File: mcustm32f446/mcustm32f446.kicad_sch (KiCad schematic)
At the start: 30 parts, among them J2 STM32WORLD_BASE, U1 AMS1117-3.3, U2 SRV05-4, U3 STM32F446RCTx, Y1 X_16MHZ

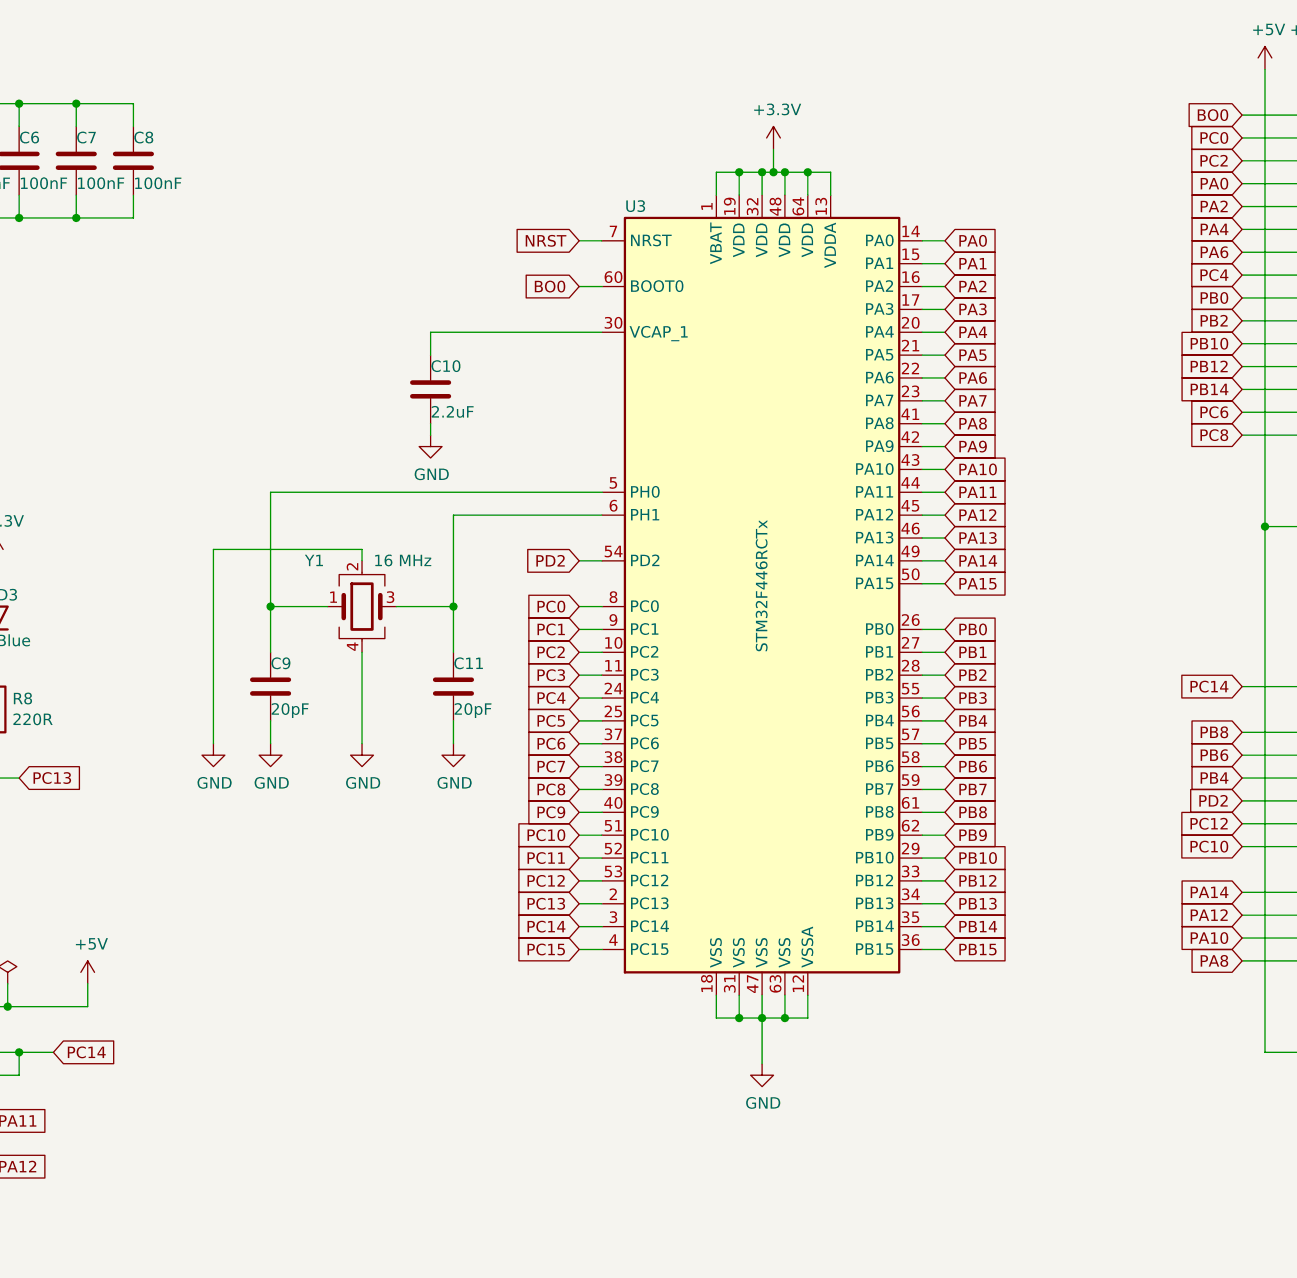
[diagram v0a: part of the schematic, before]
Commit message: Hmmmm
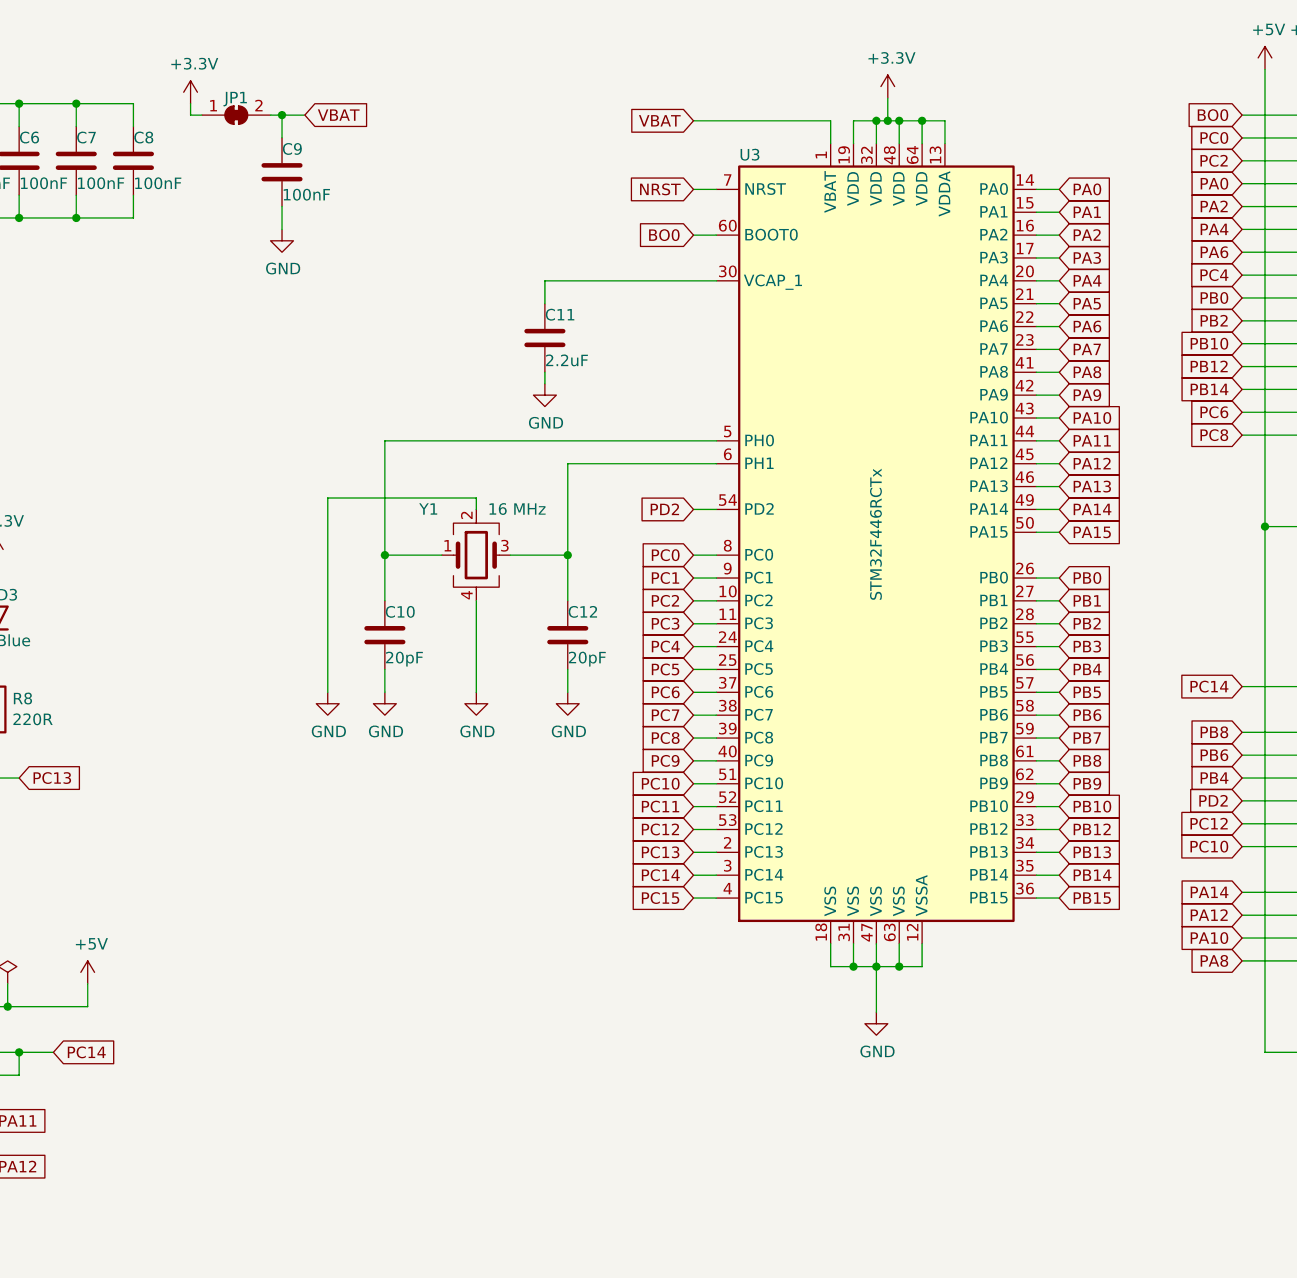
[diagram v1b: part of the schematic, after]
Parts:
- added C9: C_100NF_0603, Capacitor_SMD:C_0603_1608Metric, symbol stm32world:C_100NF_0603
- added JP1: ~, symbol Jumper:SolderJumper_2_Bridged
- renumbered C9 to C10, C10 to C11, C11 to C12
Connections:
- net +3V3: now also JP1.1 (A); no longer U3.1 (VBAT)
- net GND: now also C9.2
- new net VBAT: C9.1, JP1.2 (B), U3.1 (VBAT)
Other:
- moved on the sheet: C10, C11, C12, U3, Y1

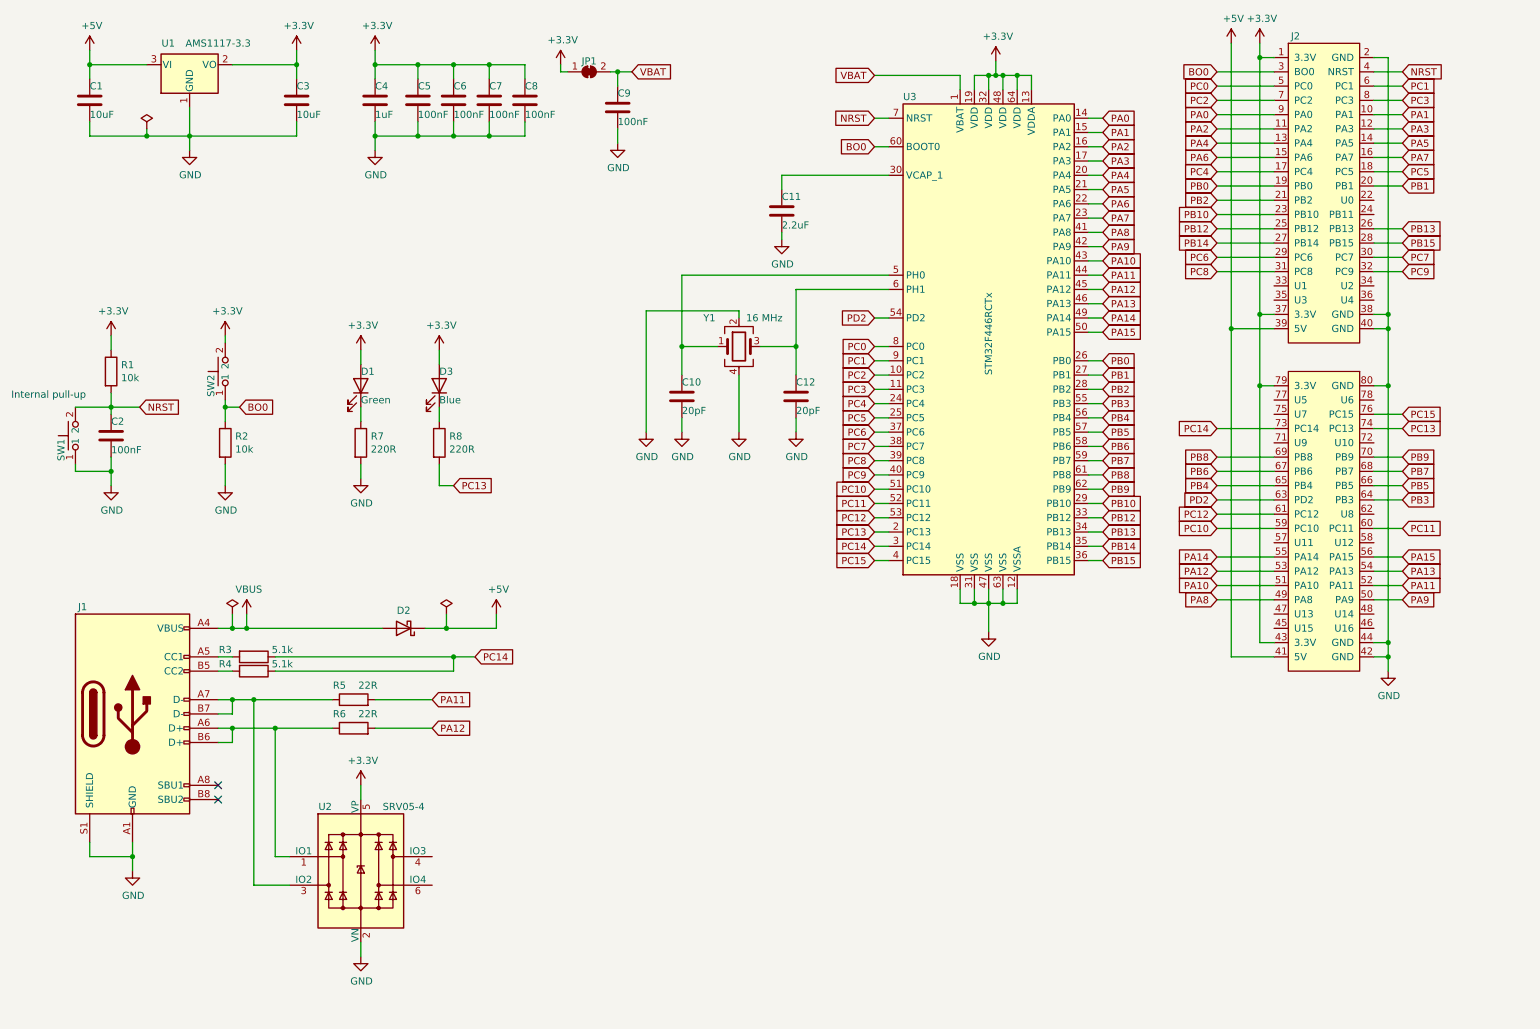
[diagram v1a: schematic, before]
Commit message: Hmmmm
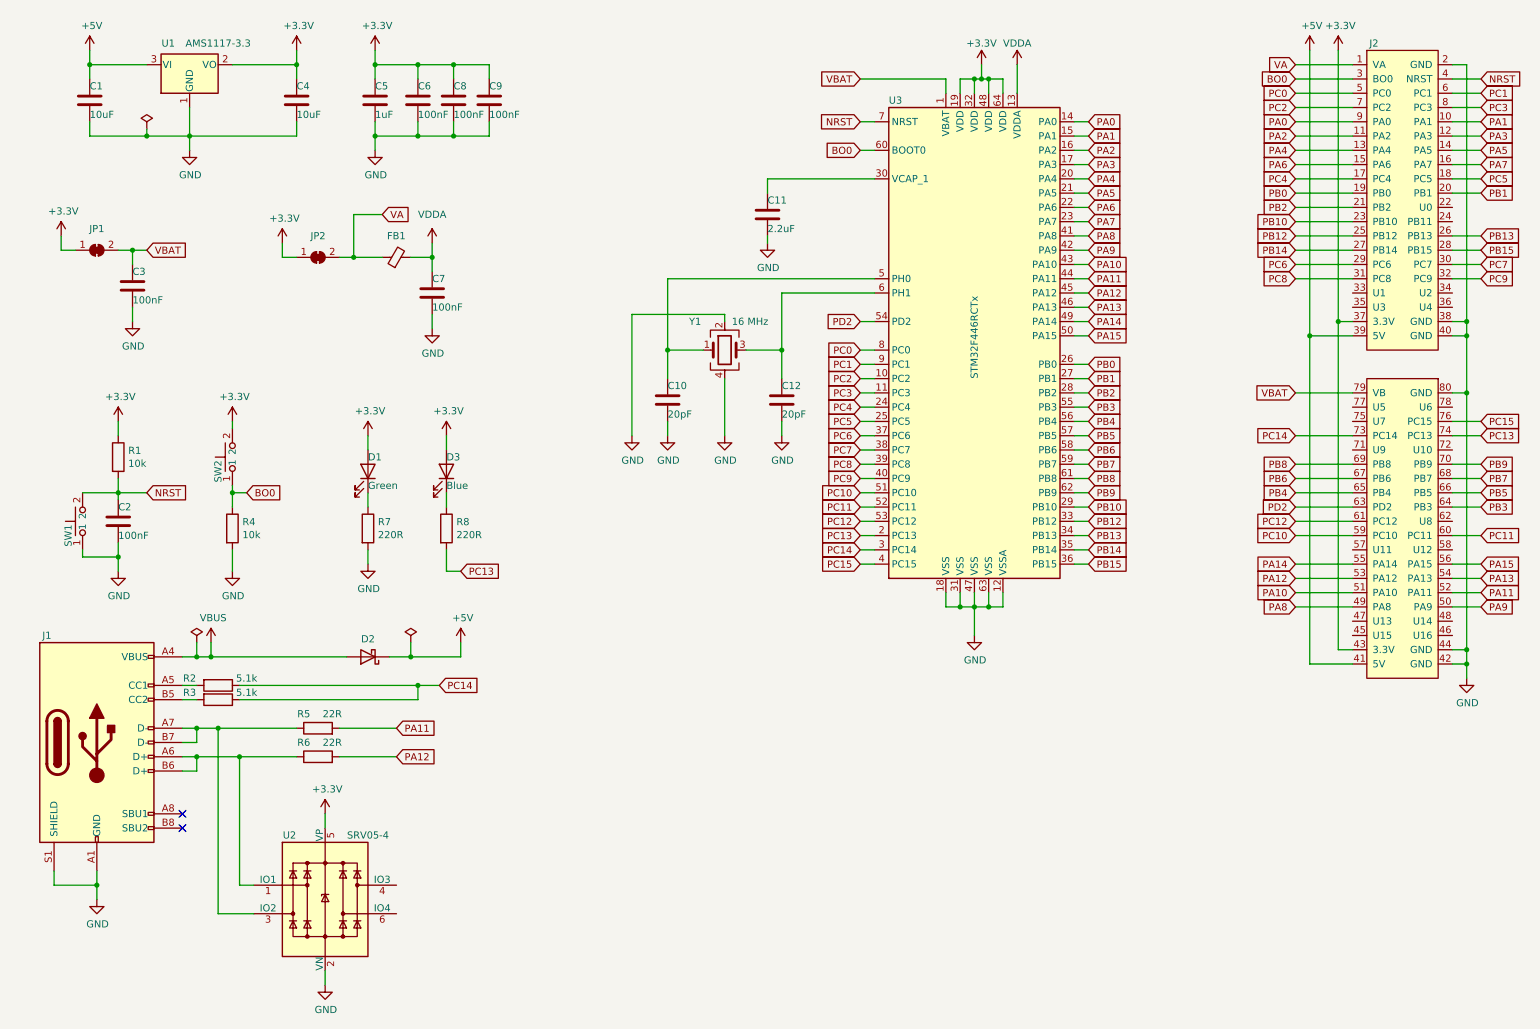
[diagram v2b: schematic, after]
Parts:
- removed JP1: ~, symbol Jumper:SolderJumper_2_Bridged
- added FB1: FB_0603, Inductor_SMD:L_0603_1608Metric, symbol stm32world:FB_0603
- added JP1, JP2: SolderJumper_2_Bridged, Jumper:SolderJumper-2_P1.3mm_Bridged_RoundedPad1.0x1.5mm, symbol stm32world:SolderJumper_2_Bridged
- renumbered C9 to C3, C3 to C4, C4 to C5, C5 to C6, C6 to C8, C8 to C9, R3 to R2, R4 to R3, R2 to R4
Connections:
- net +3V3: now also JP1.1 (A), JP2.1 (A); no longer C7.1, J2.1 (3.3V), J2.79 (3.3V), U3.13 (VDDA)
- net VBAT: now also J2.79 (VB), JP1.2 (B)
- new net VA: FB1.1, J2.1 (VA), JP2.2 (B)
- new net VDDA: C7.1, FB1.2, U3.13 (VDDA)
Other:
- note removed: "Internal pull-up"
- moved on the sheet: C10, C11, C12, C2, C3, C9, D1, D2, D3, J1, J2, R1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

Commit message: Hmmmm
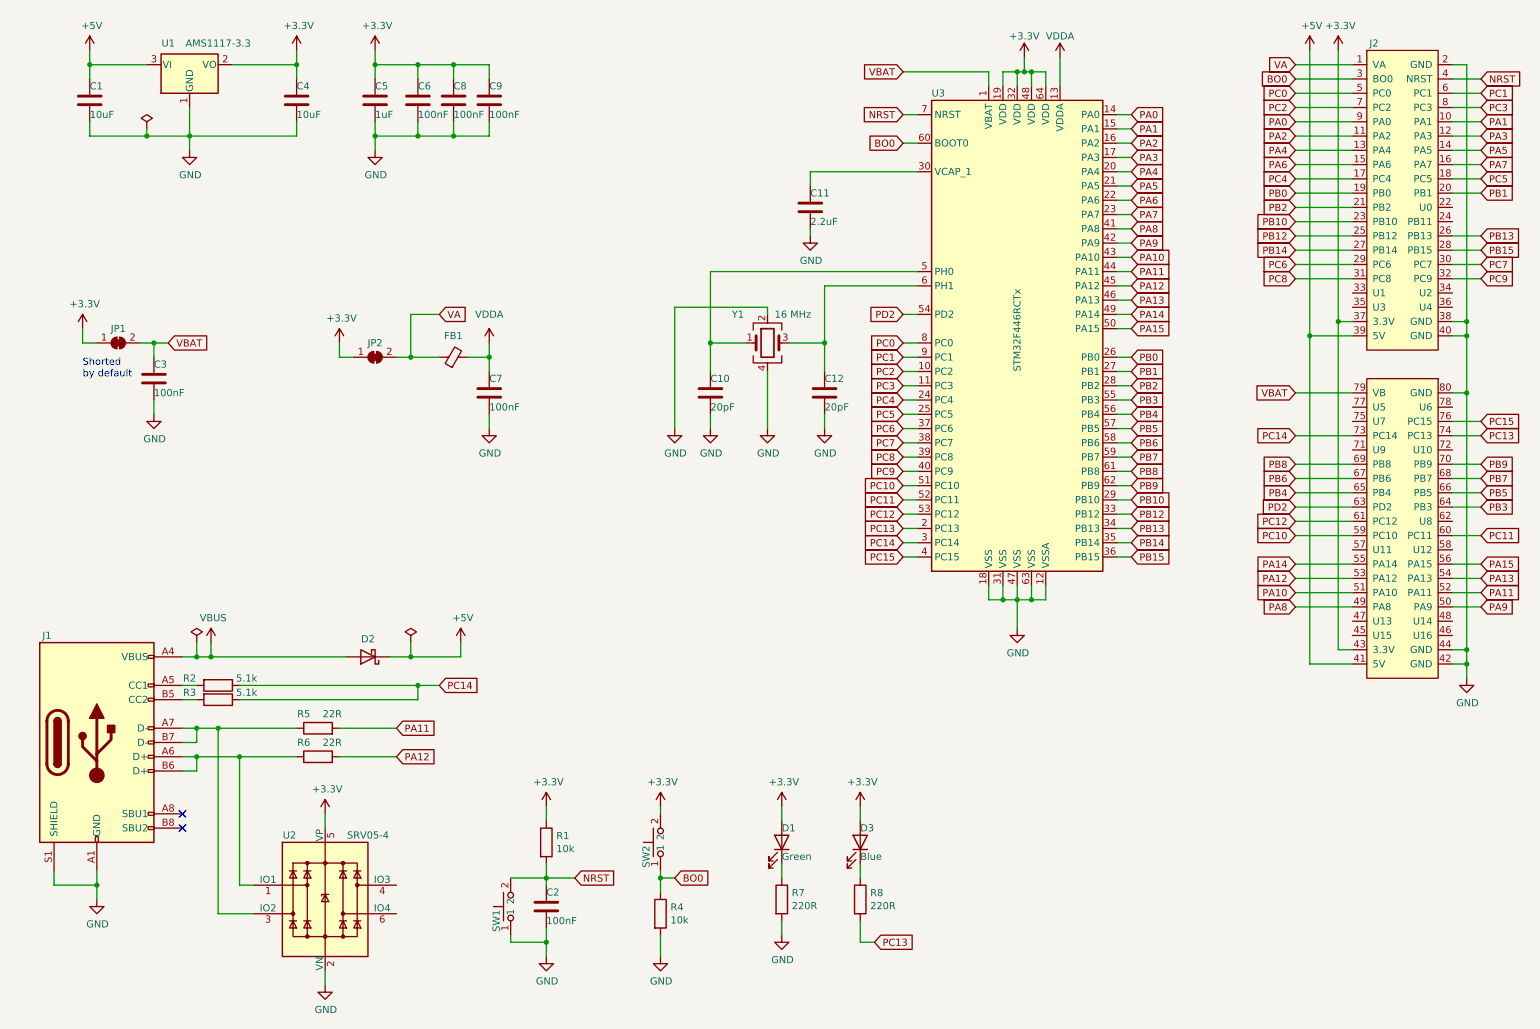
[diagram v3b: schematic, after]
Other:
- note added: "Shorted by default"
- moved on the sheet: C10, C11, C12, C2, C3, C7, D1, D3, FB1, JP1, JP2, R1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
